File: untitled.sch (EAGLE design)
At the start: 8 parts

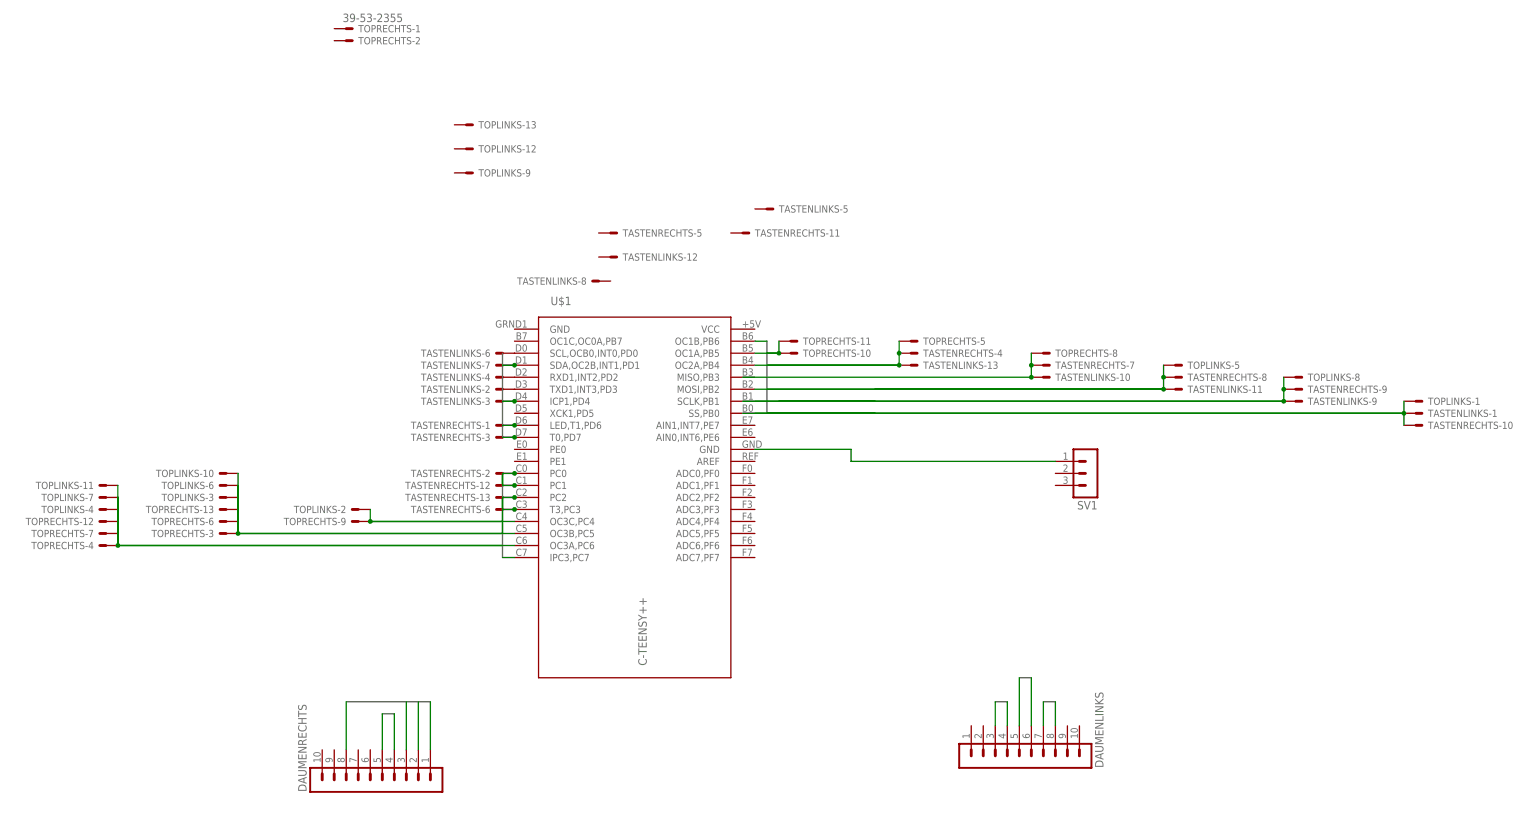
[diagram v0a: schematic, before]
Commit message: fixed wiring
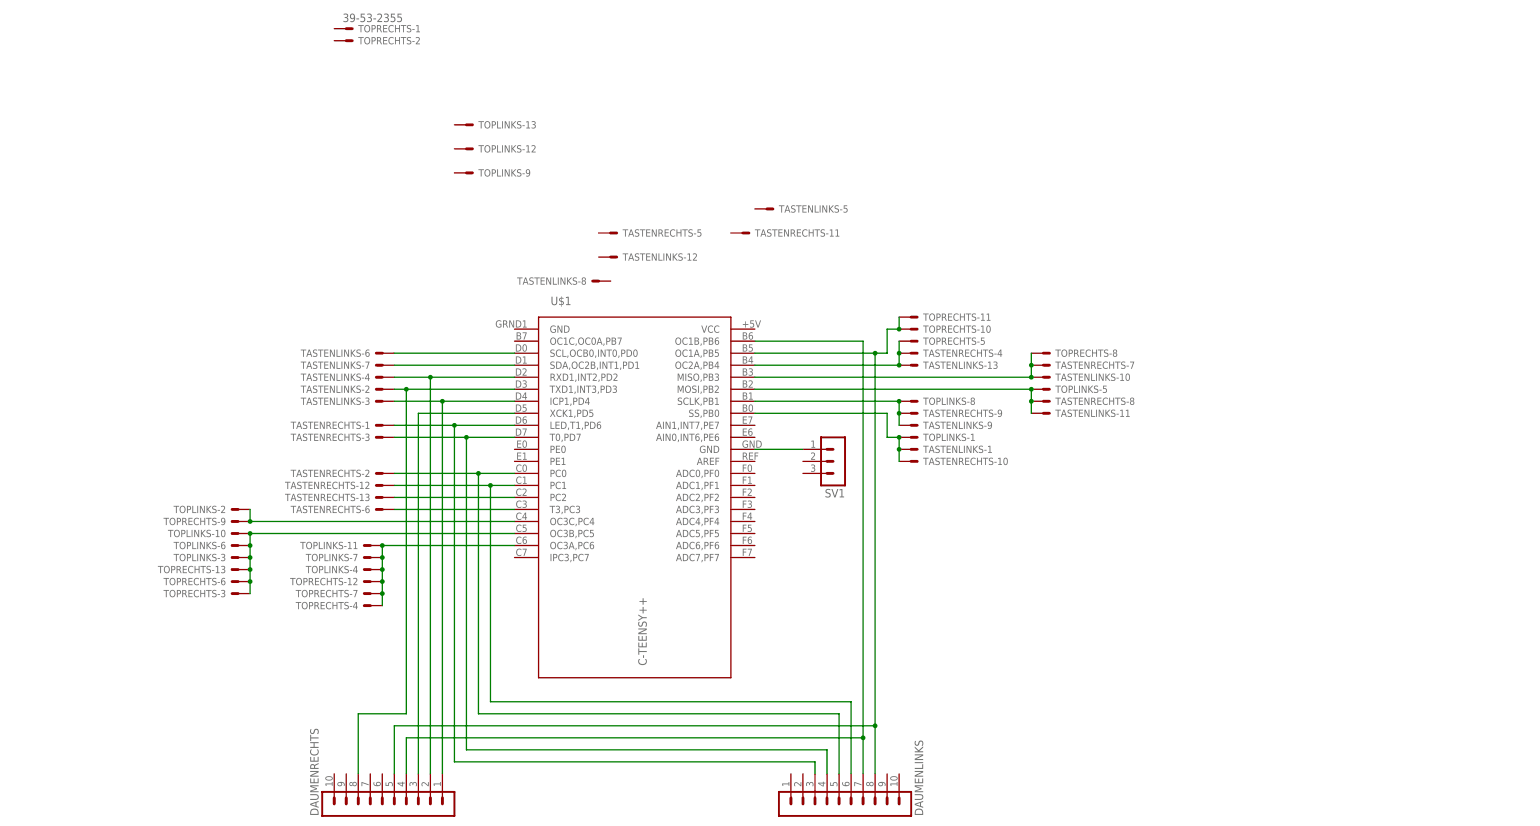
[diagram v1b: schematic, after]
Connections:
- net D1 renamed N$1
- net N$14 renamed GND
- removed net C7: U$1.IPC3,PC7
- removed net N$16: TASTENLINKS-2.S, U$1.TXD1,INT3,PD3
- removed net N$17: TASTENLINKS-4.S, U$1.RXD1,INT2,PD2
- net D2: now also TASTENLINKS-4.S, U$1.RXD1,INT2,PD2
- net D3: now also TASTENLINKS-2.S, U$1.TXD1,INT3,PD3
- net D5: now also U$1.XCK1,PD5
- net N$2: now also U$1.MISO,PB3
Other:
- moved on the sheet: DAUMENLINKS, DAUMENRECHTS, SV1, TASTENLINKS-1, TASTENLINKS-11, TASTENLINKS-2, TASTENLINKS-3, TASTENLINKS-4, TASTENLINKS-6, TASTENLINKS-7, TASTENLINKS-9, TASTENRECHTS-1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
